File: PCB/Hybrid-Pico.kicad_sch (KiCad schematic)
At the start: 39 parts, among them J1 USB_C_Receptacle_USB2.0_16P, J2 Conn_01x20, J3 Conn_01x20, J4 Conn_01x03, SW1 SW_Push, U1 RP2040, U2 MCP1700x-330xxTT, U4 W25Q16JVUXIQ TR, U5 MPU-6050, U6 BMP280, Y1 12 MHz

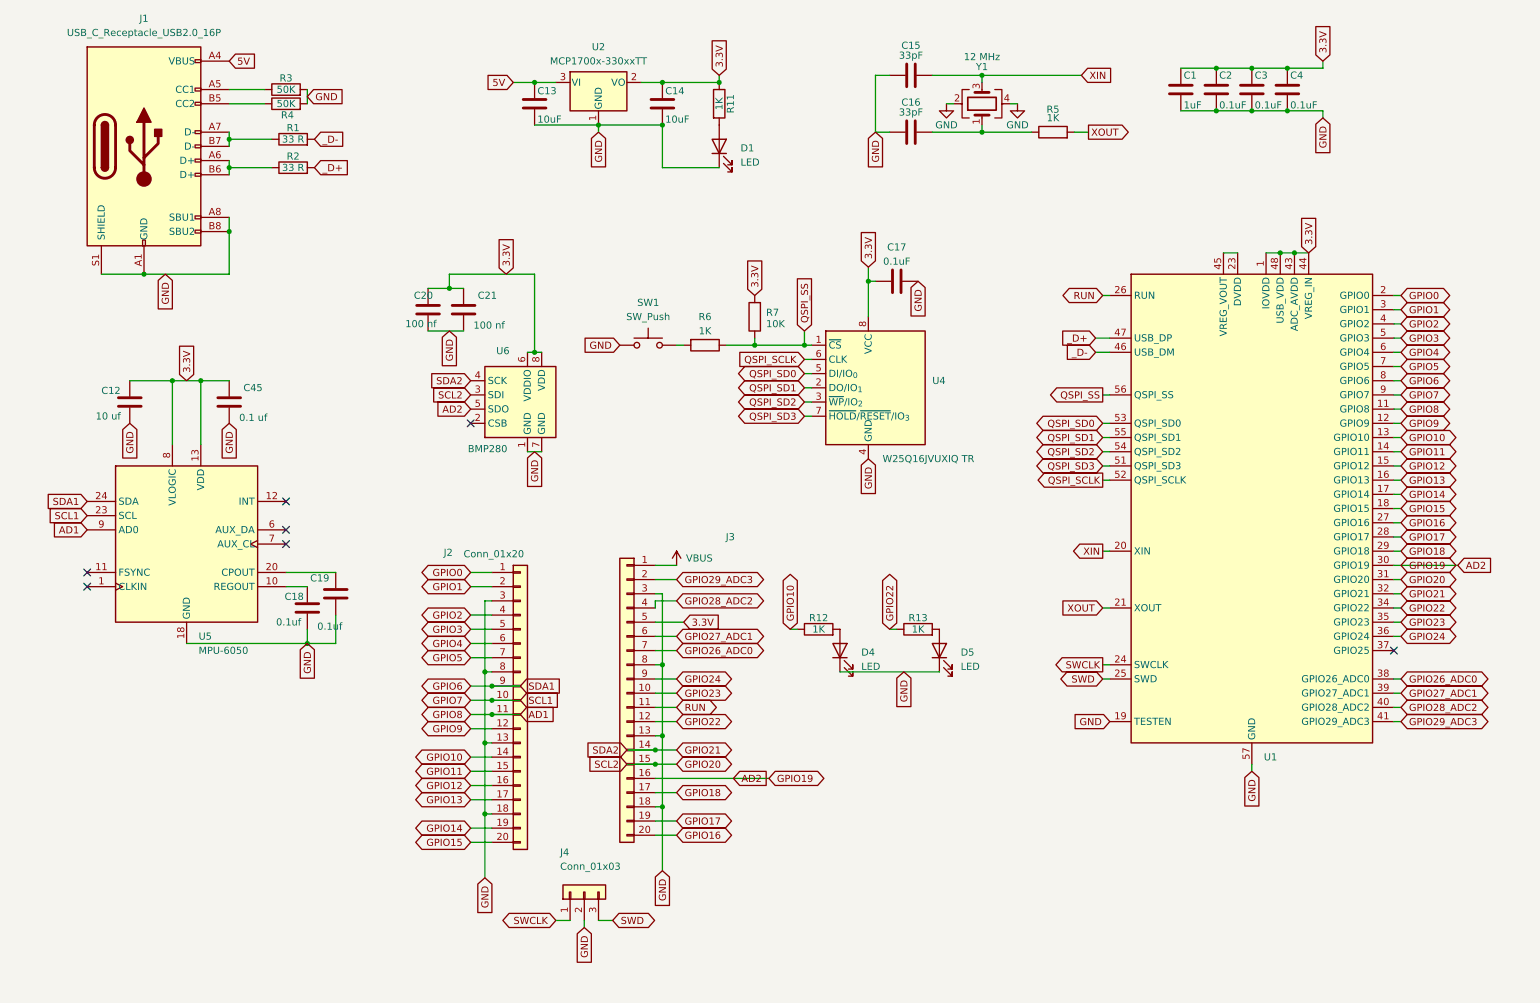
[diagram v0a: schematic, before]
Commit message: Add files via upload
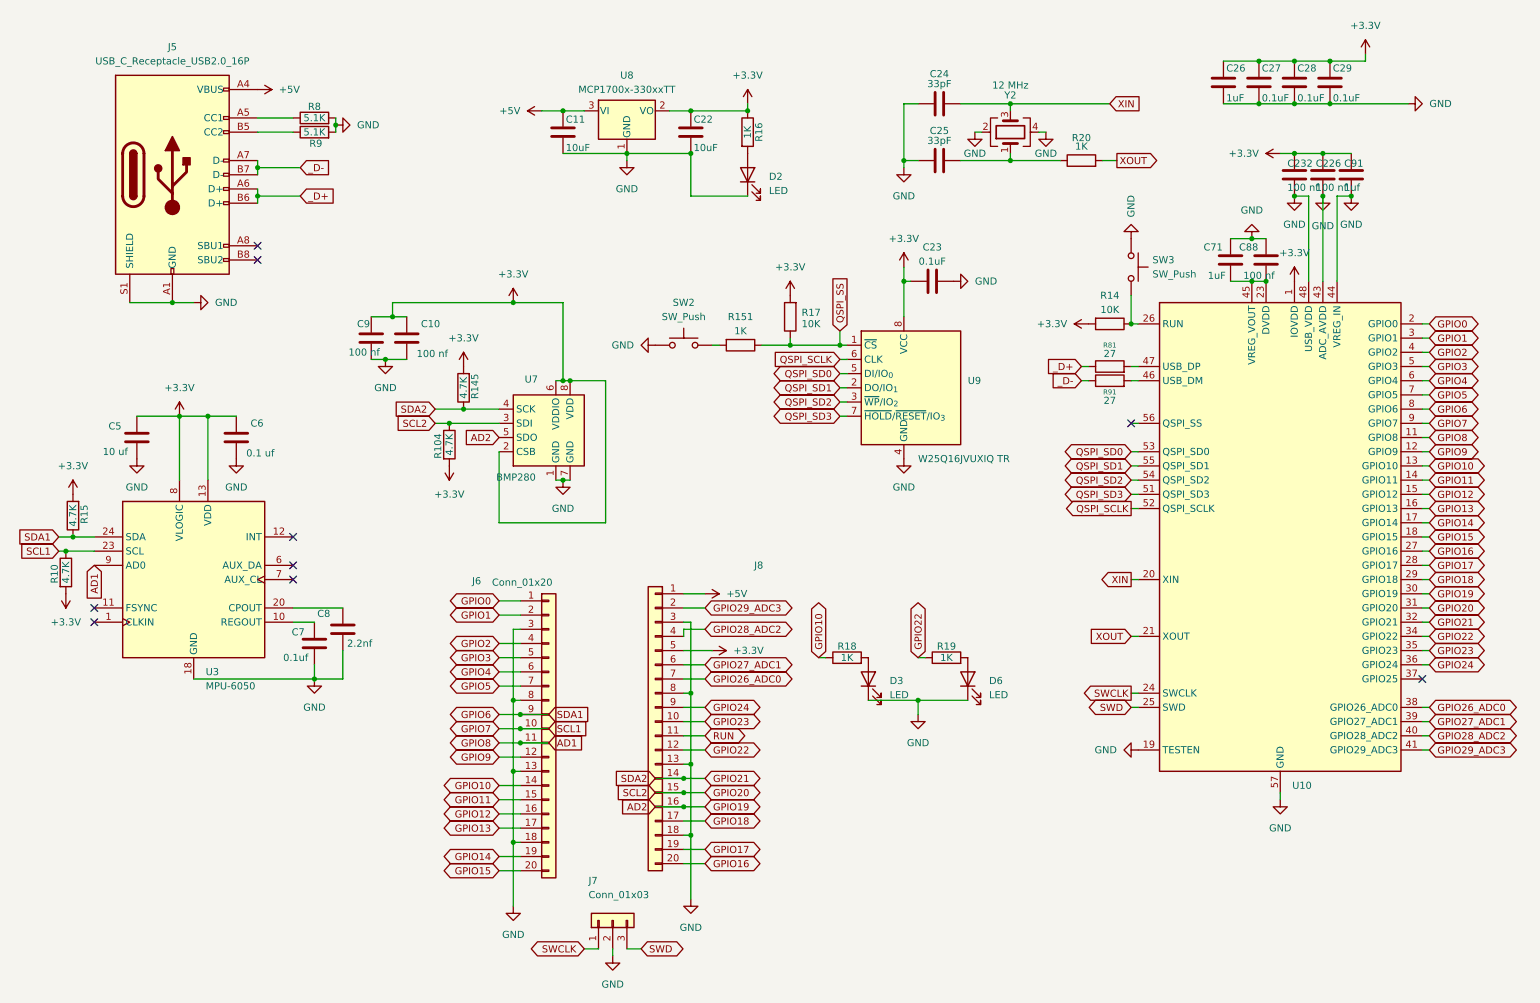
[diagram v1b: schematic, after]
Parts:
- removed C1: 1uF, Capacitor_SMD:C_0201_0603Metric, symbol Device:C
- removed C12: 10 uf, Capacitor_SMD:C_0201_0603Metric, symbol Device:C
- removed C13, C14: 10uF, Capacitor_SMD:C_0201_0603Metric, symbol Device:C
- removed C15, C16: 33pF, Capacitor_SMD:C_0201_0603Metric, symbol Device:C
- removed C17, C2, C3, C4: 0.1uF, Capacitor_SMD:C_0201_0603Metric, symbol Device:C
- removed C18, C19: 0.1uf, Capacitor_SMD:C_0201_0603Metric, symbol Device:C
- removed C20, C21: 100 nf, Capacitor_SMD:C_0201_0603Metric, symbol Device:C
- removed C45: 0.1 uf, Capacitor_SMD:C_0201_0603Metric, symbol Device:C
- removed D1, D4, D5: LED, LED_SMD:LED_0201_0603Metric, symbol Device:LED
- removed J1: USB_C_Receptacle_USB2.0_16P, Connector_USB:USB_C_Receptacle_G-Switch_GT-USB-7010ASV, symbol Connector:USB_C_Receptacle_USB2.0_16P
- removed J2, J3: Conn_01x20, Connector_PinHeader_2.54mm:PinHeader_1x20_P2.54mm_Vertical, symbol Connector_Generic:Conn_01x20
- removed J4: Conn_01x03, Connector_PinHeader_2.54mm:PinHeader_1x03_P2.54mm_Vertical, symbol Connector_Generic:Conn_01x03
- removed R1, R2: 33 R, Capacitor_SMD:C_0201_0603Metric, symbol Device:R
- removed R11, R12, R13, R5, R6: 1K, Capacitor_SMD:C_0201_0603Metric, symbol Device:R
- removed R3, R4: 50K, Capacitor_SMD:C_0201_0603Metric, symbol Device:R
- removed R7: 10K, Capacitor_SMD:C_0201_0603Metric, symbol Device:R
- removed SW1: SW_Push, Button_Switch_SMD:SW_Push_SPST_NO_Alps_SKRK, symbol Switch:SW_Push
- removed U1: RP2040, Package_DFN_QFN:QFN-56-1EP_7x7mm_P0.4mm_EP3.2x3.2mm, symbol MCU_RaspberryPi:RP2040
- removed U2: MCP1700x-330xxTT, Package_TO_SOT_SMD:SOT-23, symbol Regulator_Linear:MCP1700x-330xxTT
- removed U4: W25Q16JVUXIQ TR, Package_SON:Winbond_USON-8-1EP_3x2mm_P0.5mm_EP0.2x1.6mm, symbol Memory_Flash:W25Q16JVSS
- removed U5: MPU-6050, Sensor_Motion:InvenSense_QFN-24_4x4mm_P0.5mm, symbol Sensor_Motion:MPU-6050
- removed U6: BMP280, Package_LGA:Bosch_LGA-8_2x2.5mm_P0.65mm_ClockwisePinNumbering, symbol Sensor_Pressure:BMP280
- removed Y1: 12 MHz, Crystal:Crystal_SMD_3225-4Pin_3.2x2.5mm, symbol Device:Crystal_GND24
- added C10, C232, C9: 100 nf, Capacitor_SMD:C_0201_0603Metric, symbol Device:C
- added C11, C22: 10uF, Capacitor_SMD:C_0603_1608Metric, symbol Device:C
- added C226, C88: 100 nf, Capacitor_SMD:C_0402_1005Metric, symbol Device:C
- added C23, C27, C28, C29: 0.1uF, Capacitor_SMD:C_0603_1608Metric, symbol Device:C
- added C24, C25: 33pF, Capacitor_SMD:C_0603_1608Metric, symbol Device:C
- added C26: 1uF, Capacitor_SMD:C_0603_1608Metric, symbol Device:C
- added C5: 10 uf, Capacitor_SMD:C_0201_0603Metric, symbol Device:C
- added C6: 0.1 uf, Capacitor_SMD:C_0201_0603Metric, symbol Device:C
- added C7: 0.1uf, Capacitor_SMD:C_0201_0603Metric, symbol Device:C
- added C71: 1uF, Capacitor_SMD:C_0402_1005Metric, symbol Device:C
- added C8: 2.2nf, Capacitor_SMD:C_0201_0603Metric, symbol Device:C
- added C91: 1uf, Capacitor_SMD:C_0201_0603Metric, symbol Device:C
- added D2, D3, D6: LED, LED_SMD:LED_0201_0603Metric, symbol Device:LED
- added J5: USB_C_Receptacle_USB2.0_16P, Connector_USB:USB_C_Receptacle_G-Switch_GT-USB-7010ASV, symbol Connector:USB_C_Receptacle_USB2.0_16P
- added J6, J8: Conn_01x20, Connector_PinHeader_2.54mm:PinHeader_1x20_P2.54mm_Vertical, symbol Connector_Generic:Conn_01x20
- added J7: Conn_01x03, Connector_PinHeader_2.54mm:PinHeader_1x03_P2.54mm_Vertical, symbol Connector_Generic:Conn_01x03
- added R10, R104, R145, R15: 4.7K, Capacitor_SMD:C_0402_1005Metric, symbol Device:R
- added R14, R17: 10K, Resistor_SMD:R_0603_1608Metric, symbol Device:R
- added R151, R16, R18, R19, R20: 1K, Resistor_SMD:R_0603_1608Metric, symbol Device:R
- added R8, R9: 5.1K, Resistor_SMD:R_0603_1608Metric, symbol Device:R
- added R81, R91: 27, Capacitor_SMD:C_0402_1005Metric, symbol Device:R
- added SW2, SW3: SW_Push, Button_Switch_SMD:SW_Push_SPST_NO_Alps_SKRK, symbol Switch:SW_Push
- added U10: RP2040, Package_DFN_QFN:QFN-56-1EP_7x7mm_P0.4mm_EP3.2x3.2mm, symbol MCU_RaspberryPi:RP2040
- added U3: MPU-6050, Sensor_Motion:InvenSense_QFN-24_4x4mm_P0.5mm, symbol Sensor_Motion:MPU-6050
- added U7: BMP280, Package_LGA:Bosch_LGA-8_2x2.5mm_P0.65mm_ClockwisePinNumbering, symbol Sensor_Pressure:BMP280
- added U8: MCP1700x-330xxTT, Package_TO_SOT_SMD:SOT-23, symbol Regulator_Linear:MCP1700x-330xxTT
- added U9: W25Q16JVUXIQ TR, Package_SON:Winbond_USON-8-1EP_3x2mm_P0.5mm_EP0.2x1.6mm, symbol Memory_Flash:W25Q16JVSS
- added Y2: 12 MHz, Crystal:Crystal_SMD_3225-4Pin_3.2x2.5mm, symbol Device:Crystal_GND24
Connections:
- net AD1: now also J6.11 (Pin_11), U10.11 (GPIO8), U3.9 (AD0)
- net AD2: now also J8.16 (Pin_16), U10.30 (GPIO19), U7.5 (SDO)
- net GND: now also C10.2, C11.2, C22.2, C226.2, C23.2, C232.2, C24.1, C25.1, C26.2, C27.2, C28.2, C29.2, C5.2, C6.2, C7.2, C71.1, C8.2, C88.1, C9.2, C91.2, D2.1 (K), D3.1 (K), D6.1 (K), J5.A1 (GND), J5.A12 (GND), J5.B1 (GND), J5.B12 (GND), J5.S1 (SHIELD), J6.13 (Pin_13), J6.18 (Pin_18), J6.3 (Pin_3), J6.8 (Pin_8), J7.2 (Pin_2), J8.13 (Pin_13), J8.18 (Pin_18), J8.3 (Pin_3), J8.8 (Pin_8), R8.2, R9.2, SW2.1, SW3.1, U10.19 (TESTEN), U10.43 (ADC_AVDD), U10.44 (VREG_IN), U10.48 (USB_VDD), U10.57 (GND), U3.18 (GND), U7.1 (GND), U7.7 (GND), U8.1 (GND), U9.4 (GND), Y2.2, Y2.4
- net GPIO0: now also J6.1 (Pin_1), U10.2 (GPIO0)
- net GPIO1: now also J6.2 (Pin_2), U10.3 (GPIO1)
- net GPIO10: now also J6.14 (Pin_14), R18.1, U10.13 (GPIO10)
- net GPIO11: now also J6.15 (Pin_15), U10.14 (GPIO11)
- net GPIO12: now also J6.16 (Pin_16), U10.15 (GPIO12)
- net GPIO13: now also J6.17 (Pin_17), U10.16 (GPIO13)
- net GPIO14: now also J6.19 (Pin_19), U10.17 (GPIO14)
- net GPIO15: now also J6.20 (Pin_20), U10.18 (GPIO15)
- net GPIO16: now also J8.20 (Pin_20), U10.27 (GPIO16)
- net GPIO17: now also J8.19 (Pin_19), U10.28 (GPIO17)
- net GPIO18: now also J8.17 (Pin_17), U10.29 (GPIO18)
- net GPIO2: now also J6.4 (Pin_4), U10.4 (GPIO2)
- net GPIO20: now also J8.15 (Pin_15), R104.1, U10.31 (GPIO20), U7.3 (SDI)
- net GPIO21: now also J8.14 (Pin_14), R145.1, U10.32 (GPIO21), U7.4 (SCK)
- net GPIO22: now also J8.12 (Pin_12), R19.1, U10.34 (GPIO22)
- net GPIO23: now also J8.10 (Pin_10), U10.35 (GPIO23)
- net GPIO24: now also J8.9 (Pin_9), U10.36 (GPIO24)
- net GPIO26_ADC0: now also J8.7 (Pin_7), U10.38 (GPIO26_ADC0)
- net GPIO27_ADC1: now also J8.6 (Pin_6), U10.39 (GPIO27_ADC1)
- net GPIO28_ADC2: now also J8.4 (Pin_4), U10.40 (GPIO28_ADC2)
- net GPIO29_ADC3: now also J8.2 (Pin_2), U10.41 (GPIO29_ADC3)
- net GPIO3: now also J6.5 (Pin_5), U10.5 (GPIO3)
- net GPIO4: now also J6.6 (Pin_6), U10.6 (GPIO4)
- net GPIO5: now also J6.7 (Pin_7), U10.7 (GPIO5)
- net GPIO6: now also J6.9 (Pin_9), R15.1, U10.8 (GPIO6), U3.24 (SDA)
- net GPIO7: now also J6.10 (Pin_10), R10.1, U10.9 (GPIO7), U3.23 (SCL)
- net GPIO9: now also J6.12 (Pin_12), U10.12 (GPIO9)
- net QSPI_SCLK: now also U10.52 (QSPI_SCLK), U9.6 (CLK)
- net QSPI_SD0: now also U10.53 (QSPI_SD0), U9.5 (DI/IO_{0})
- net QSPI_SD1: now also U10.55 (QSPI_SD1), U9.2 (DO/IO_{1})
- net QSPI_SD2: now also U10.54 (QSPI_SD2), U9.3 (~{WP}/IO_{2})
- net QSPI_SD3: now also U10.51 (QSPI_SD3), U9.7 (~{HOLD}/~{RESET}/IO_{3})
- net QSPI_SS: now also R151.1, R17.1, U9.1 (~{CS})
- net RUN: now also J8.11 (Pin_11)
- net SWCLK: now also J7.1 (Pin_1), U10.24 (SWCLK)
- net SWD: now also J7.3 (Pin_3), U10.25 (SWD)
- net XIN: now also C24.2, U10.20 (XIN), Y2.3
- net XOUT: now also R20.2, U10.21 (XOUT)
- net _D+: now also J5.A6 (D+), J5.B6 (D+), R81.1
- net _D-: now also J5.A7 (D-), J5.B7 (D-), R91.1
- new net: C71.2, C88.2, U10.23 (DVDD), U10.45 (VREG_VOUT), U10.50 (DVDD)
- new net: J5.A5 (CC1), R8.1
- new net: J5.B5 (CC2), R9.1
- new net: D2.2 (A), R16.2
- new net: D6.2 (A), R19.2
- new net: C8.1, U3.20 (CPOUT)
- new net: C25.2, R20.1, Y2.1
- new net: R14.1, SW3.2, U10.26 (RUN)
- new net: D3.2 (A), R18.2
- new net: R151.2, SW2.2
- new net: C7.1, U3.10 (REGOUT)
- new net: R91.2, U10.46 (USB_DM)
- new net: R81.2, U10.47 (USB_DP)
- new net +3.3V: C10.1, C22.1, C226.1, C23.1, C232.1, C26.1, C27.1, C28.1, C29.1, C5.1, C6.1, C9.1, C91.1, J8.5 (Pin_5), R10.2, R104.2, R14.2, R145.2, R15.2, R16.1, R17.2, U10.1 (IOVDD), U10.10 (IOVDD), U10.22 (IOVDD), U10.33 (IOVDD), U10.42 (IOVDD), U10.49 (IOVDD), U3.13 (VDD), U3.8 (VLOGIC), U7.2 (CSB), U7.6 (VDDIO), U7.8 (VDD), U8.2 (VO), U9.8 (VCC)
- new net +5V: C11.1, J5.A4 (VBUS), J5.A9 (VBUS), J5.B4 (VBUS), J5.B9 (VBUS), J8.1 (Pin_1), U8.3 (VI)
- no-connect marks 7 -> 9
